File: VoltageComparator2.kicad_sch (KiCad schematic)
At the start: 6 parts, among them U18 LM324, U19 74LS08

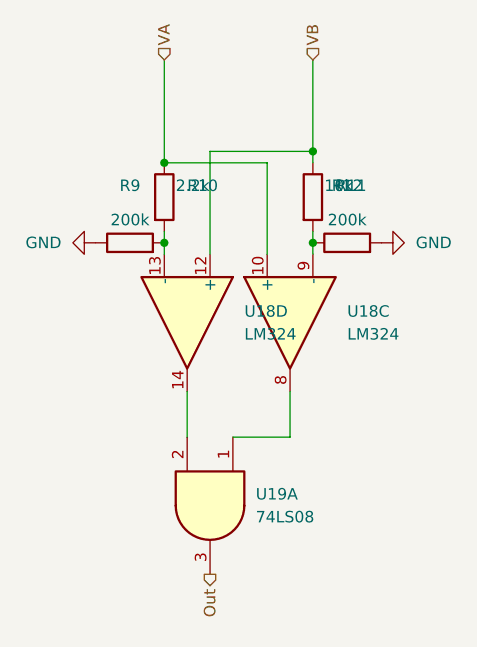
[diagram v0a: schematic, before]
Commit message: Ground and Power Plane?
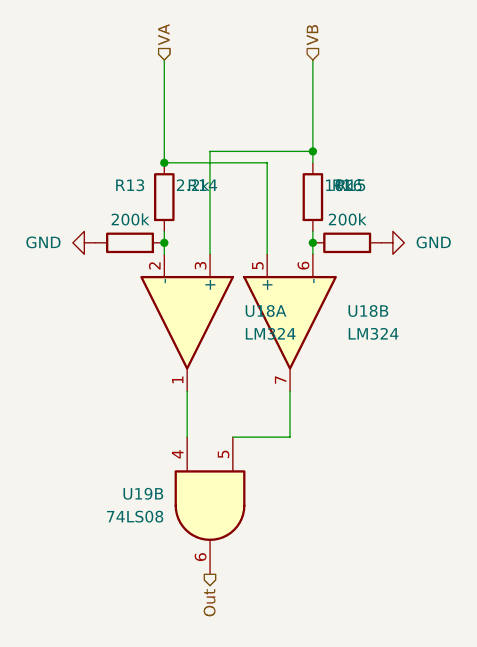
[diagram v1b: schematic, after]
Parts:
- renumbered R9 to R13, R10 to R14, R11 to R15, R12 to R16
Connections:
- net Out: now also U19.6; no longer U19.3
- net VA: now also U18.5 (+); no longer U18.10 (+)
- net VB: now also U18.3 (+); no longer U18.12 (+)
- net at R13.2, R14.2: now also U18.2 (-); no longer U18.13 (-)
- net at R15.2, R16.1: now also U18.6 (-); no longer U18.9 (-)
- new net: U18.1, U19.4
- new net: U18.7, U19.5
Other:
- moved on the sheet: U19B
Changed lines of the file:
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@@
 	(symbol
 		(lib_id "74xx:74LS08")
-		(at 53.34 96.52 270)
-		(unit 1)
+		(at 53.34 96.52 90)
+		(mirror x)
+		(unit 2)
 		(exclude_from_sim no)
 		(in_bom yes)
@@
 		(dnp no)
 		(property "Reference" "U19"
-			(at 58.42 95.2416 90)
+			(at 48.26 95.2416 90)
 			(effects
 				(font
@@
 		)
 		(property "Value" "74LS08"
-			(at 58.42 97.7816 90)
+			(at 48.26 97.7816 90)
 			(effects
 				(font
@@
 		(dnp no)
 		(fields_autoplaced yes)
-		(property "Reference" "#PWR088"
+		(property "Reference" "#PWR090"
 			(at 78.74 67.31 0)
 			(effects
@@
 		(instances
 			(project "ECE145Mastermind"
-				(path "/8c64fe8a-5d6b-41bc-b3a3-9bda7b2e0f2c/4f59e726-7fd4-4ef0-8dbb-7a41976aa953"
-					(reference "#PWR088")
+				(path "/8c64fe8a-5d6b-41bc-b3a3-9bda7b2e0f2c/acb554fe-df67-46ea-bc1c-079edbbfc216"
+					(reference "#PWR090")
 					(unit 1)
 				)
@@
 		(on_board yes)
 		(dnp no)
-		(property "Reference" "R10"
+		(property "Reference" "R14"
 			(at 50.8 60.9599 0)
 			(effects
@@
 		(instances
 			(project "ECE145Mastermind"
-				(path "/8c64fe8a-5d6b-41bc-b3a3-9bda7b2e0f2c/4f59e726-7fd4-4ef0-8dbb-7a41976aa953"
-					(reference "R10")
+				(path "/8c64fe8a-5d6b-41bc-b3a3-9bda7b2e0f2c/acb554fe-df67-46ea-bc1c-079edbbfc216"
+					(reference "R14")
 					(unit 1)
 				)
@@
 		(dnp no)
 		(fields_autoplaced yes)
-		(property "Reference" "#PWR087"
+		(property "Reference" "#PWR089"
 			(at 34.29 67.31 0)
 			(effects
@@
 		(instances
 			(project "ECE145Mastermind"
-				(path "/8c64fe8a-5d6b-41bc-b3a3-9bda7b2e0f2c/4f59e726-7fd4-4ef0-8dbb-7a41976aa953"
-					(reference "#PWR087")
+				(path "/8c64fe8a-5d6b-41bc-b3a3-9bda7b2e0f2c/acb554fe-df67-46ea-bc1c-079edbbfc216"
+					(reference "#PWR089")
 					(unit 1)
 				)
@@
 		(on_board yes)
 		(dnp no)
-		(property "Reference" "R11"
+		(property "Reference" "R15"
 			(at 67.31 60.9599 0)
 			(effects
@@
 		(instances
 			(project "ECE145Mastermind"
-				(path "/8c64fe8a-5d6b-41bc-b3a3-9bda7b2e0f2c/4f59e726-7fd4-4ef0-8dbb-7a41976aa953"
-					(reference "R11")
+				(path "/8c64fe8a-5d6b-41bc-b3a3-9bda7b2e0f2c/acb554fe-df67-46ea-bc1c-079edbbfc216"
+					(reference "R15")
 					(unit 1)
 				)
@@
 		(at 62.23 76.2 90)
 		(mirror x)
-		(unit 3)
+		(unit 2)
 		(exclude_from_sim no)
 		(in_bom yes)
@@
 		(instances
 			(project "ECE145Mastermind"
-				(path "/8c64fe8a-5d6b-41bc-b3a3-9bda7b2e0f2c/4f59e726-7fd4-4ef0-8dbb-7a41976aa953"
+				(path "/8c64fe8a-5d6b-41bc-b3a3-9bda7b2e0f2c/acb554fe-df67-46ea-bc1c-079edbbfc216"
 					(reference "U18")
-					(unit 3)
+					(unit 2)
 				)
 			)
@@
 		(lib_id "Amplifier_Operational:LM324")
 		(at 50.8 76.2 270)
-		(unit 4)
+		(unit 1)
 		(exclude_from_sim no)
 		(in_bom yes)
@@
 		(instances
 			(project "ECE145Mastermind"
-				(path "/8c64fe8a-5d6b-41bc-b3a3-9bda7b2e0f2c/4f59e726-7fd4-4ef0-8dbb-7a41976aa953"
+				(path "/8c64fe8a-5d6b-41bc-b3a3-9bda7b2e0f2c/acb554fe-df67-46ea-bc1c-079edbbfc216"
 					(reference "U18")
-					(unit 4)
+					(unit 1)
 				)
 			)
@@
 		(on_board yes)
 		(dnp no)
-		(property "Reference" "R9"
+		(property "Reference" "R13"
 			(at 44.45 60.96 90)
 			(effects
@@
 		(instances
 			(project "ECE145Mastermind"
-				(path "/8c64fe8a-5d6b-41bc-b3a3-9bda7b2e0f2c/4f59e726-7fd4-4ef0-8dbb-7a41976aa953"
-					(reference "R9")
+				(path "/8c64fe8a-5d6b-41bc-b3a3-9bda7b2e0f2c/acb554fe-df67-46ea-bc1c-079edbbfc216"
+					(reference "R13")
 					(unit 1)
 				)
@@
 		(on_board yes)
 		(dnp no)
-		(property "Reference" "R12"
+		(property "Reference" "R16"
 			(at 68.58 60.96 90)
 			(effects
@@
 		(instances
 			(project "ECE145Mastermind"
-				(path "/8c64fe8a-5d6b-41bc-b3a3-9bda7b2e0f2c/4f59e726-7fd4-4ef0-8dbb-7a41976aa953"
-					(reference "R12")
-					(unit 1)
-				)
+				(path "/8c64fe8a-5d6b-41bc-b3a3-9bda7b2e0f2c/acb554fe-df67-46ea-bc1c-079edbbfc216"
+					(reference "R16")
+					(unit 1)
+				)

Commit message: Finished?
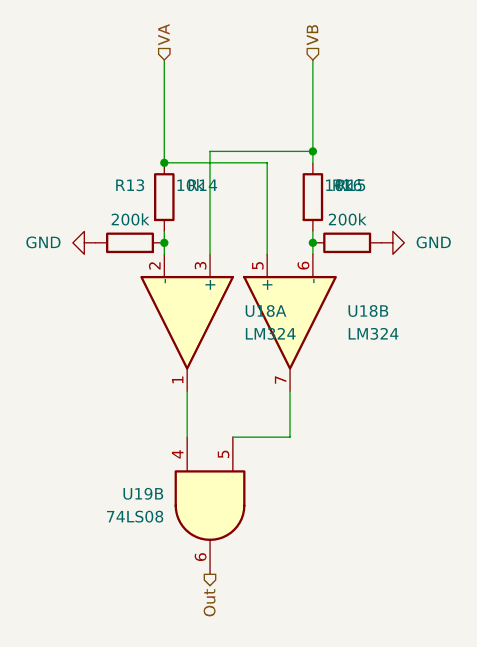
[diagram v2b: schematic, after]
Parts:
- R14: value 2.2k -> 10k
